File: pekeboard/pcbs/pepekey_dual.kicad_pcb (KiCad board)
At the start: 2 copper layers, 148.5 x 124.9 mm, 63 parts

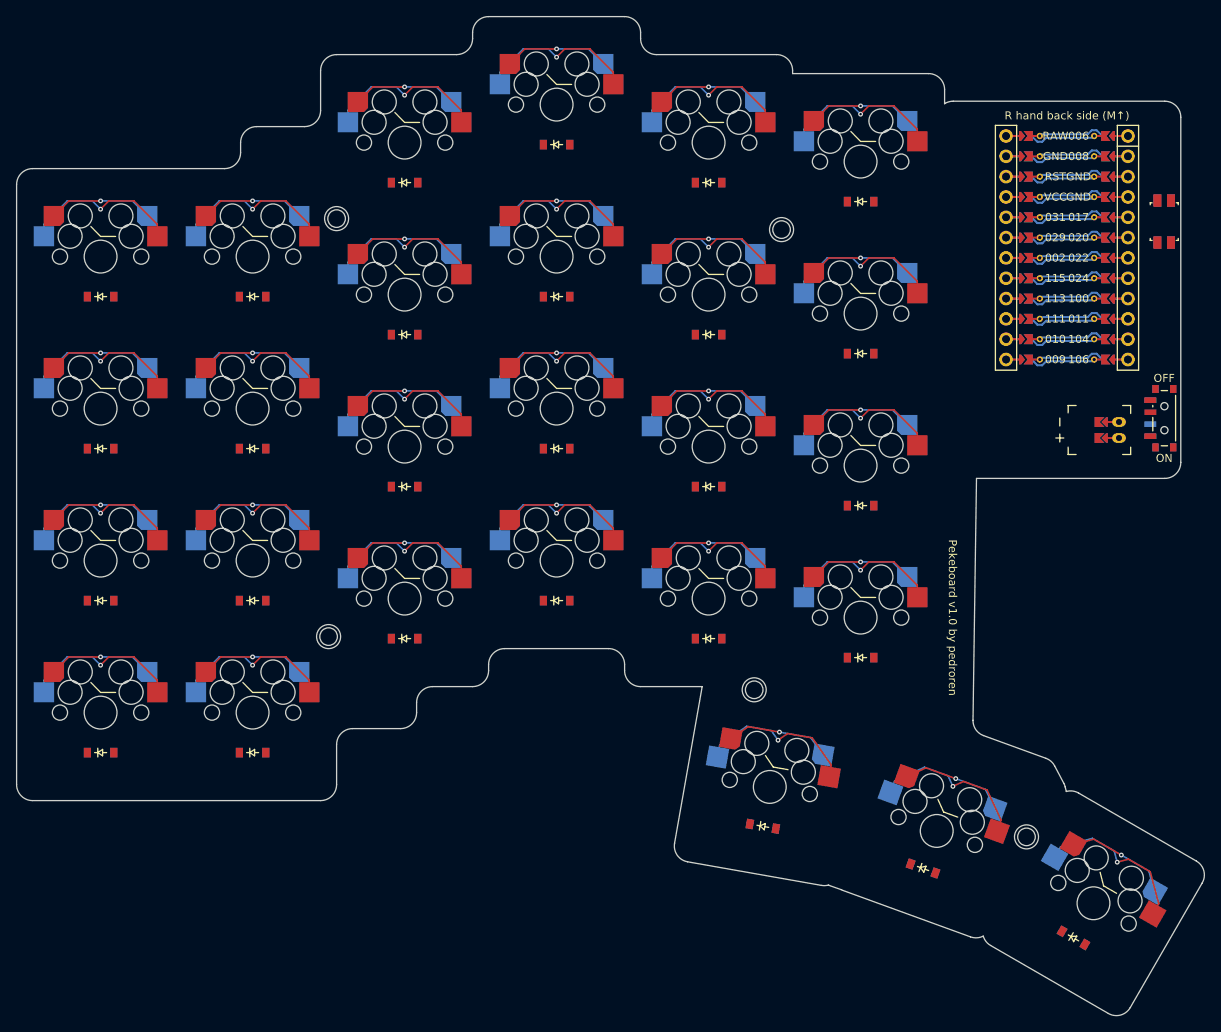
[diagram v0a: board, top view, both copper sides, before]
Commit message: cleanup and built zmk firmware files
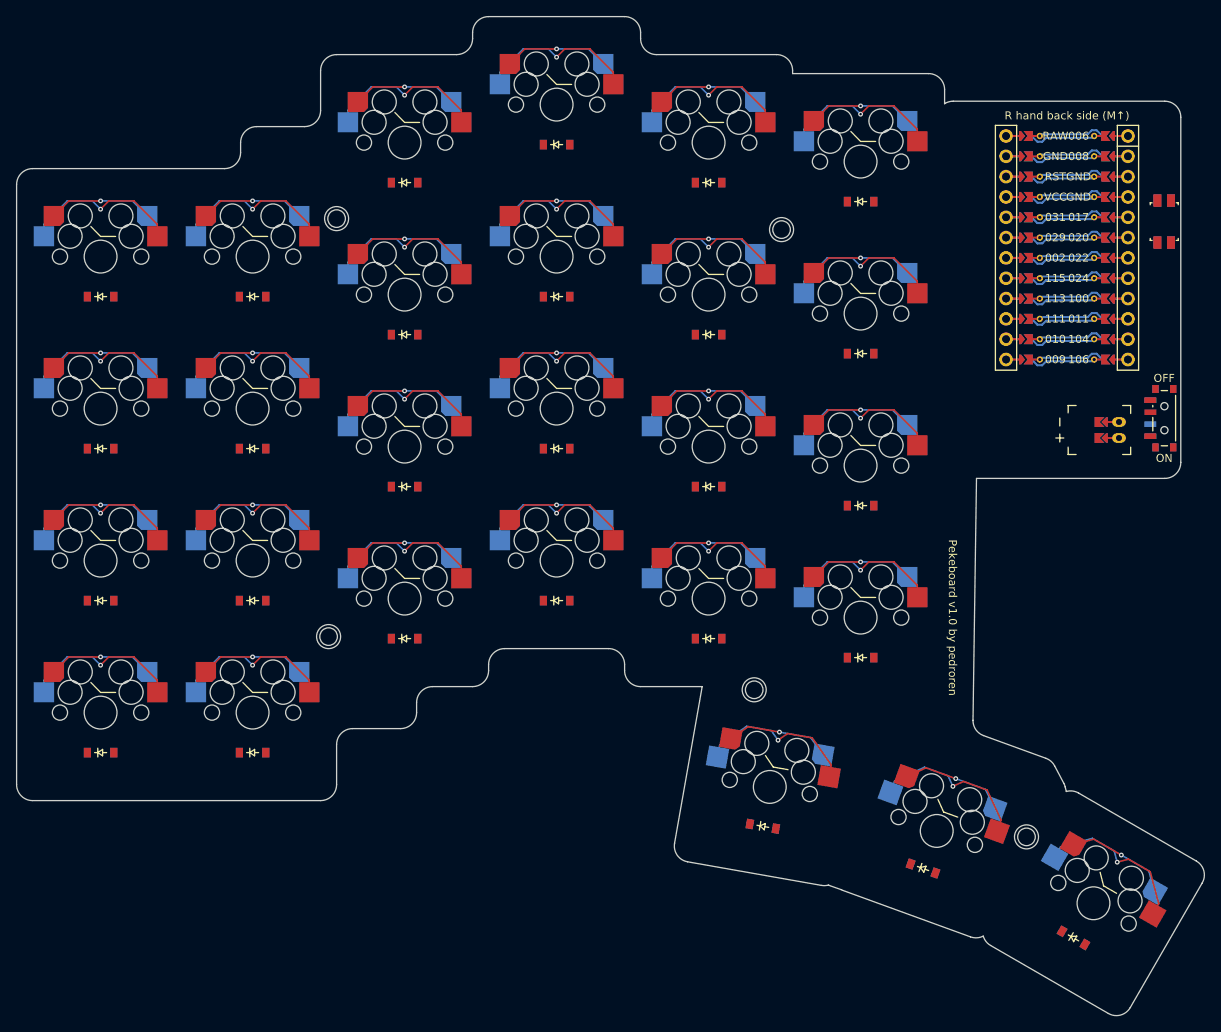
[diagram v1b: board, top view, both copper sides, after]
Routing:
- net (no net): track 0.00 -> 337.7 mm
- net P106: track 112.0 -> 52.9 mm
- net P011: track 112.0 -> 52.9 mm
- net P100: track 91.6 -> 42.3 mm
- net P024: track 91.6 -> 42.3 mm
- net P008: track 91.6 -> 42.3 mm
- net P022: track 91.6 -> 42.3 mm
- net GND: track 29.5 -> 0.00 mm
- net P111: track 30.3 -> 10.6 mm
- net inner_thumbrow: track 13.2 -> 23.1 mm
- net ring_num: track 13.2 -> 23.1 mm
- net middle_top: track 13.2 -> 23.1 mm
- net middle_num: track 13.2 -> 23.1 mm
- net inner_num: track 13.2 -> 23.1 mm
- net index_num: track 13.2 -> 23.1 mm
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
